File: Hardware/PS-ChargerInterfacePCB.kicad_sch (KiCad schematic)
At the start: 31 parts, among them J1 ElconConn, J2 SFH11-PBPC-D05-ST-BK, J3 BPSConn, J5 Estop 3, J8 EVSE Conn, J9 CarCANConnector, U1 LeaderSOM

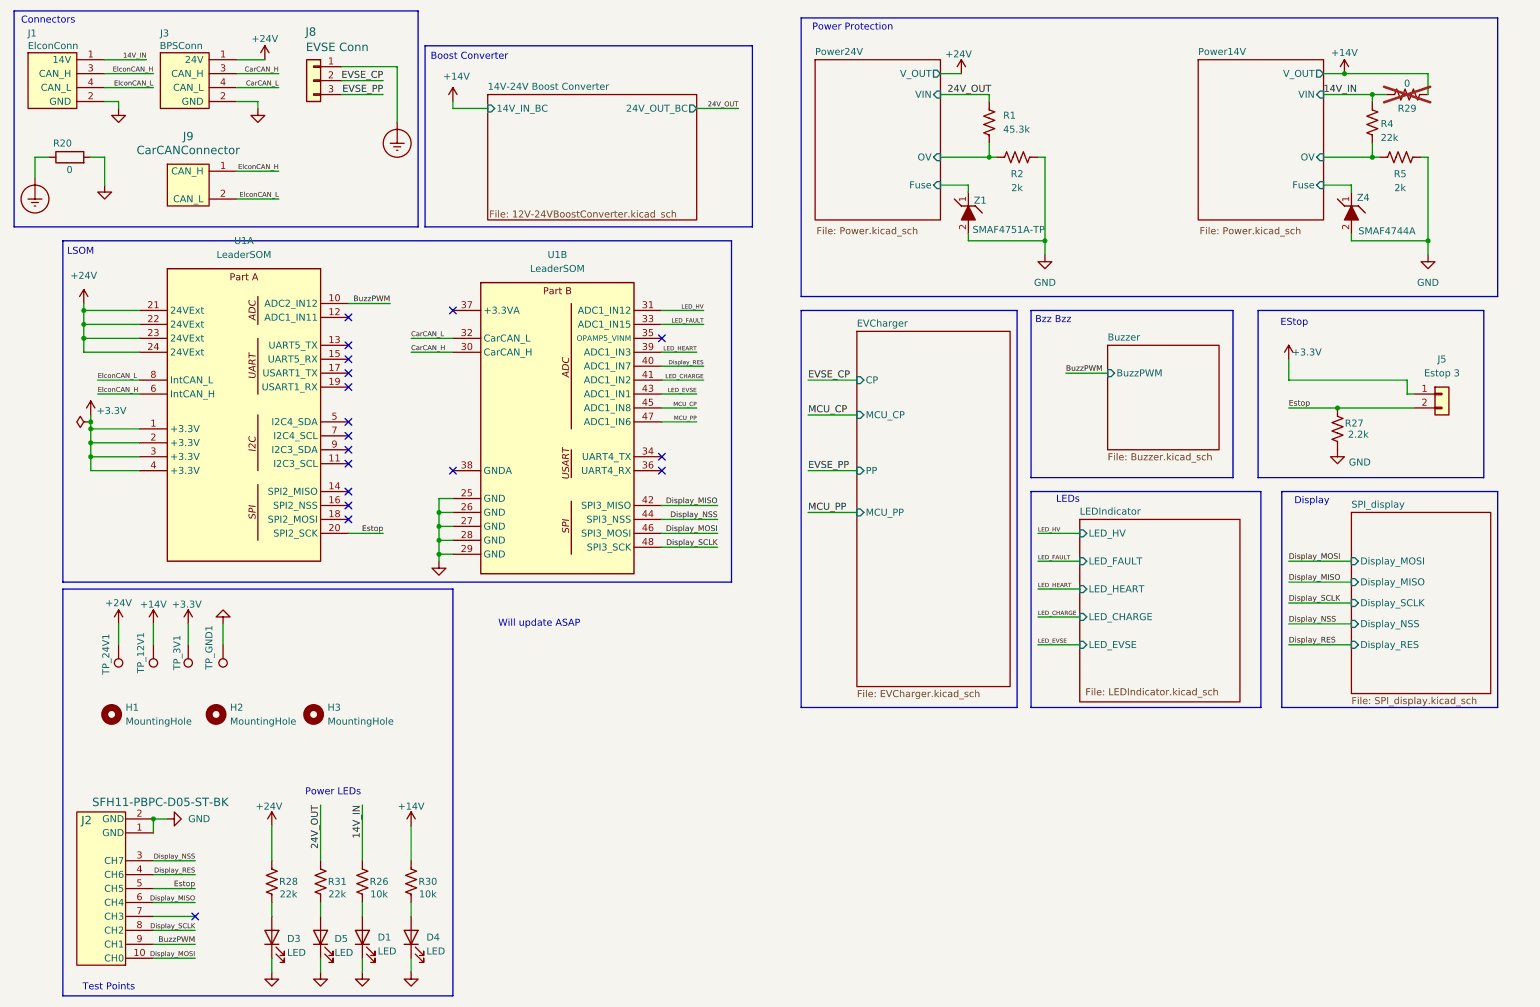
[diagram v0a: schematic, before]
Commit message: Review council
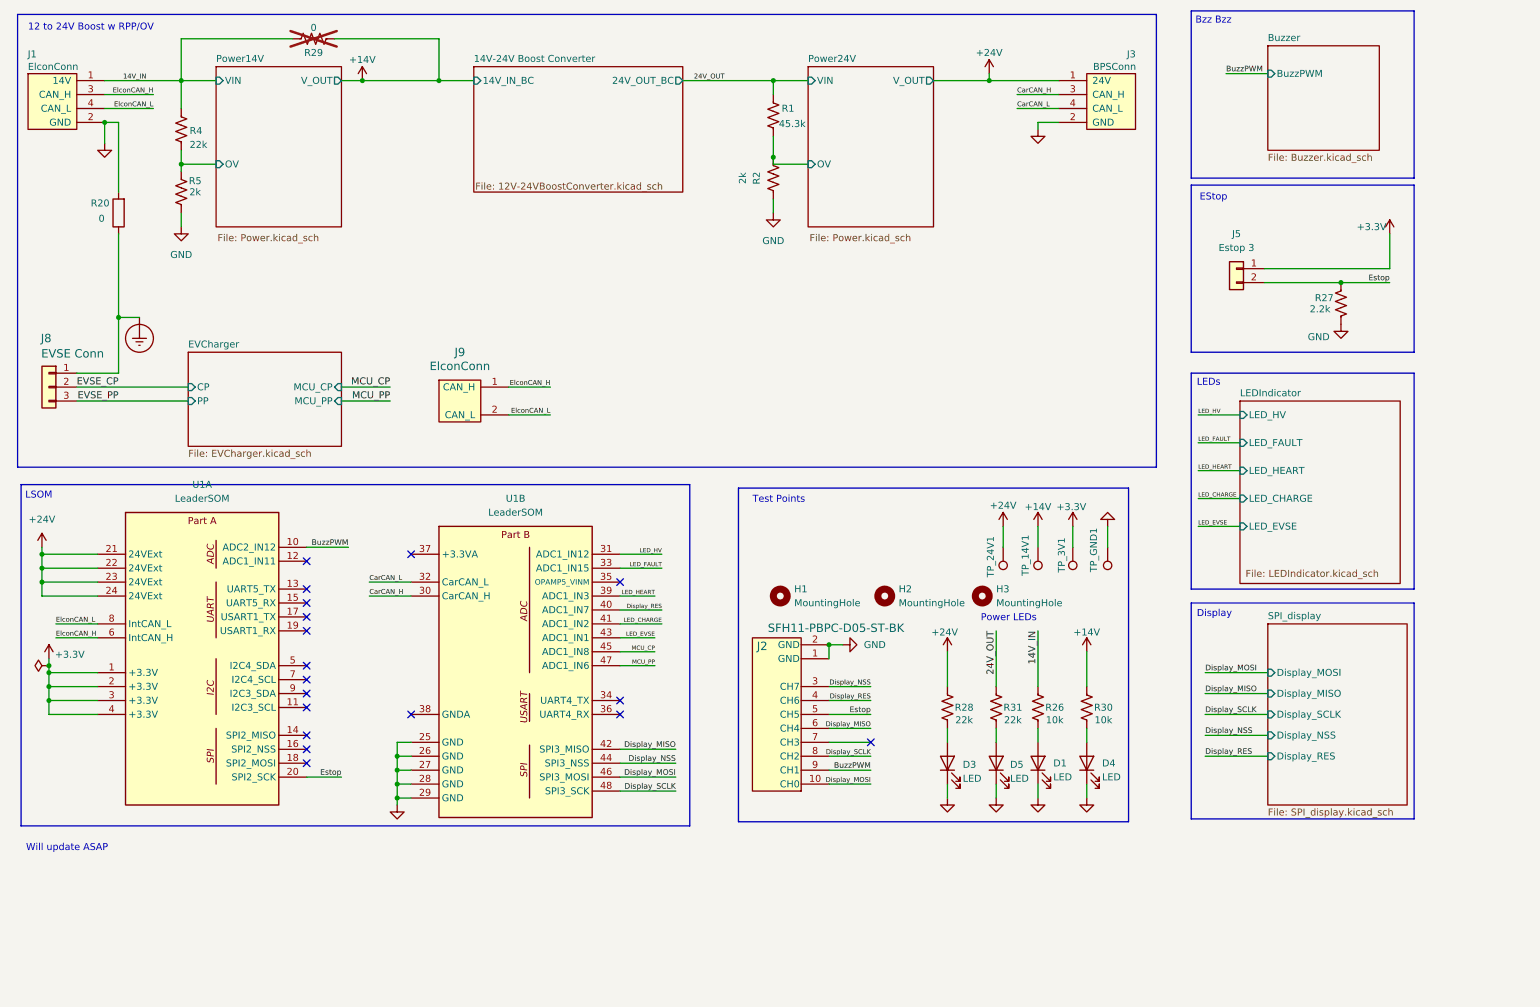
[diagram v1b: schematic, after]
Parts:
- removed Z1: SMAF4751A-TP, UTSVT_Passives:SODFL5026X125N, symbol UTSVT_Power:SMAF4749A-TP
- removed Z4: SMAF4744A, UTSVT_Passives:SODFL5026X125N, symbol UTSVT_Power:SMAF4749A-TP
- J9: value CarCANConnector -> ElconConn
- renumbered TP_12V1 to TP_14V1
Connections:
- net GND: now also R5.1; no longer R5.2
- net Power14V/OV: now also R5.2; no longer R5.1
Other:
- sheet Power14V ports: added none; removed Fuse
- sheet Power24V ports: added none; removed Fuse
- note added: "12 to 24V Boost w RPP/OV"
- note removed: "Boost Converter"
- note removed: "Connectors"
- note removed: "Power Protection"
- moved on the sheet: D1, D3, D4, D5, H1, H2, H3, J1, J2, J3, J5, J8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
